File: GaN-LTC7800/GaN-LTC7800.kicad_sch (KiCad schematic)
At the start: 27 parts, among them Q1 EPC2066, Q2 EPC2066, U1 LTC7800HUDC_PBF

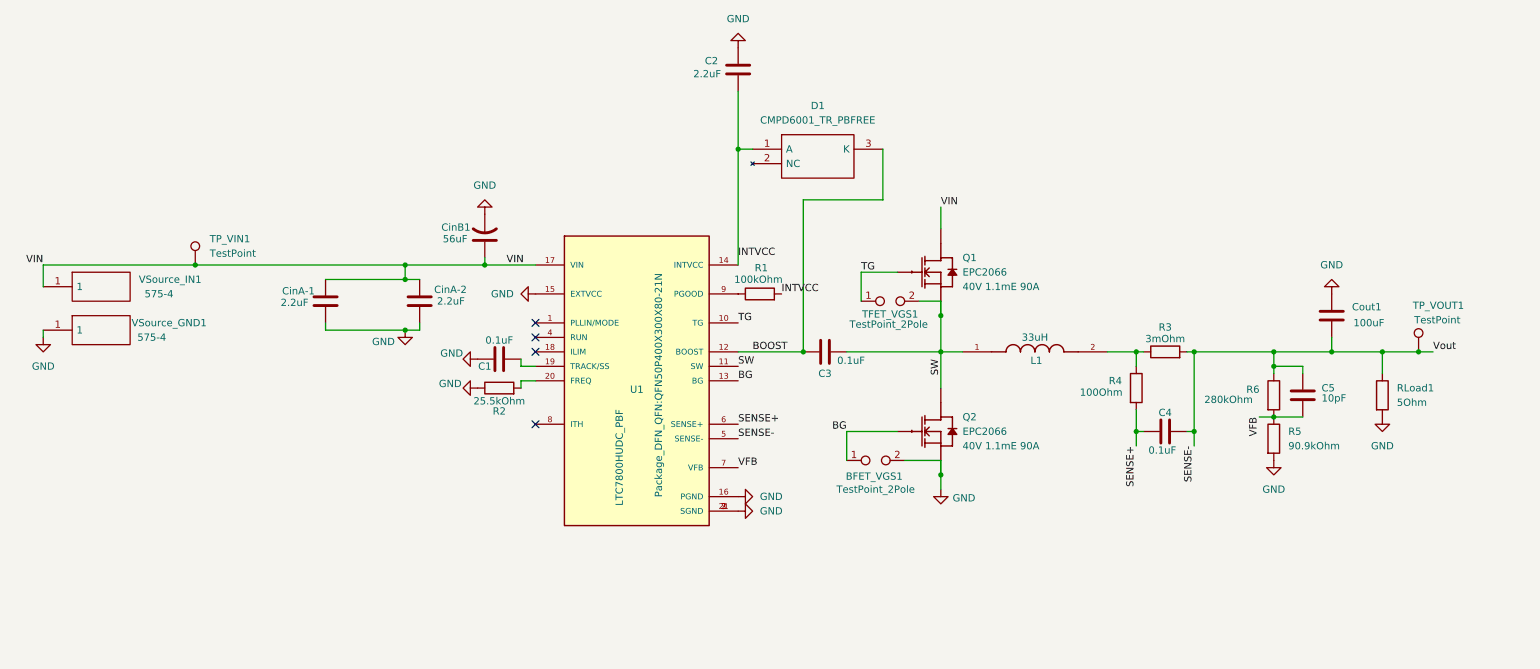
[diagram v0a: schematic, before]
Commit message: Updated shematics
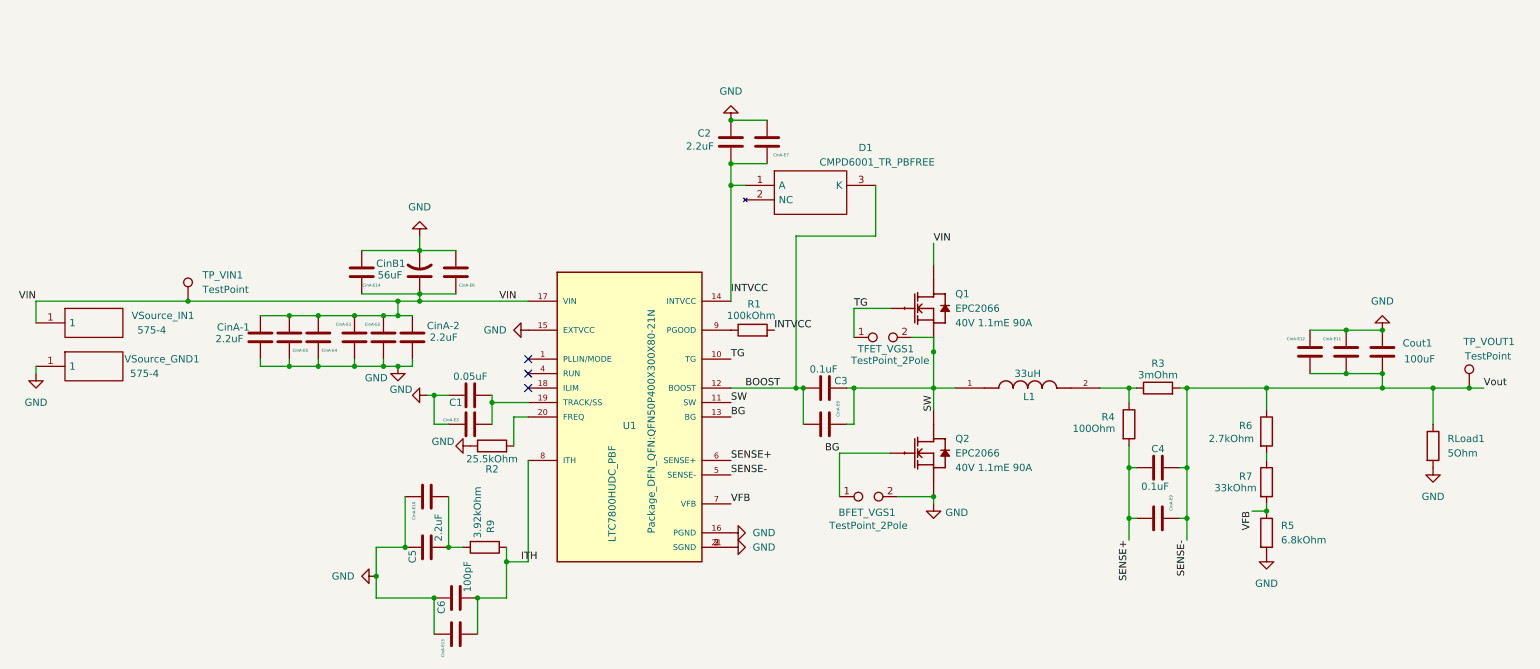
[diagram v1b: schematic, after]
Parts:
- added C6: 100pF, Capacitor_SMD:C_0805_2012Metric_Pad1.18x1.45mm_HandSolder, symbol Device:C
- added CinA-E1, CinA-E10, CinA-E11, CinA-E12, CinA-E13, CinA-E14, CinA-E2, CinA-E3, CinA-E4, CinA-E5, CinA-E6, CinA-E7, CinA-E8, CinA-E9: ~, Capacitor_SMD:C_0805_2012Metric_Pad1.18x1.45mm_HandSolder, symbol Device:C
- added R7: 33kOhm, Resistor_SMD:R_0201_0603Metric_Pad0.64x0.40mm_HandSolder, symbol Device:R
- added R9: 3.92kOhm, Resistor_SMD:R_0201_0603Metric_Pad0.64x0.40mm_HandSolder, symbol Device:R
- C1: value 0.1uF -> 0.05uF
- C5: value 10pF -> 2.2uF
- R5: value 90.9kOhm -> 6.8kOhm
- R6: value 280kOhm -> 2.7kOhm
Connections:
- net BOOST: now also CinA-E8.2
- net GND: now also C5.1, C6.1, CinA-E1.2, CinA-E10.1, CinA-E11.1, CinA-E12.1, CinA-E13.1, CinA-E14.2, CinA-E2.2, CinA-E3.1, CinA-E4.1, CinA-E5.1, CinA-E6.2, CinA-E7.2
- net INTVCC: now also CinA-E7.1
- net SENSE+: now also CinA-E9.2
- net SENSE-: now also CinA-E11.2, CinA-E12.2, CinA-E9.1; no longer C5.1
- net SW: now also CinA-E8.1
- net VFB: now also R7.2; no longer C5.2, R6.2
- net VIN: now also CinA-E1.1, CinA-E14.1, CinA-E2.1, CinA-E4.2, CinA-E5.2, CinA-E6.1
- net at C1.2, U1.19 (TRACK/SS): now also CinA-E3.2
- net ITH: now reaches U1.8 (ITH)
- net ITH: now also C6.2, CinA-E13.2, R9.1
- new net: C5.2, CinA-E10.2, R9.2
- new net: R6.2, R7.1
- no-connect marks 4 -> 3
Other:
- moved on the sheet: BFET_VGS1, C1, C2, C3, C4, C5, CinA-1, CinA-2, CinB1, Cout1, D1, L1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
